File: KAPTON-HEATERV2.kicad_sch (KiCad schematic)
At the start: 21 parts, among them J1 XT60PW-M, J2 XT60PW-M, J3 1985276, J4 1985218, J5 10090926-P154XLF, K1 1-1393210-8, Q1 AO3400A, U1 TC4427ACOA

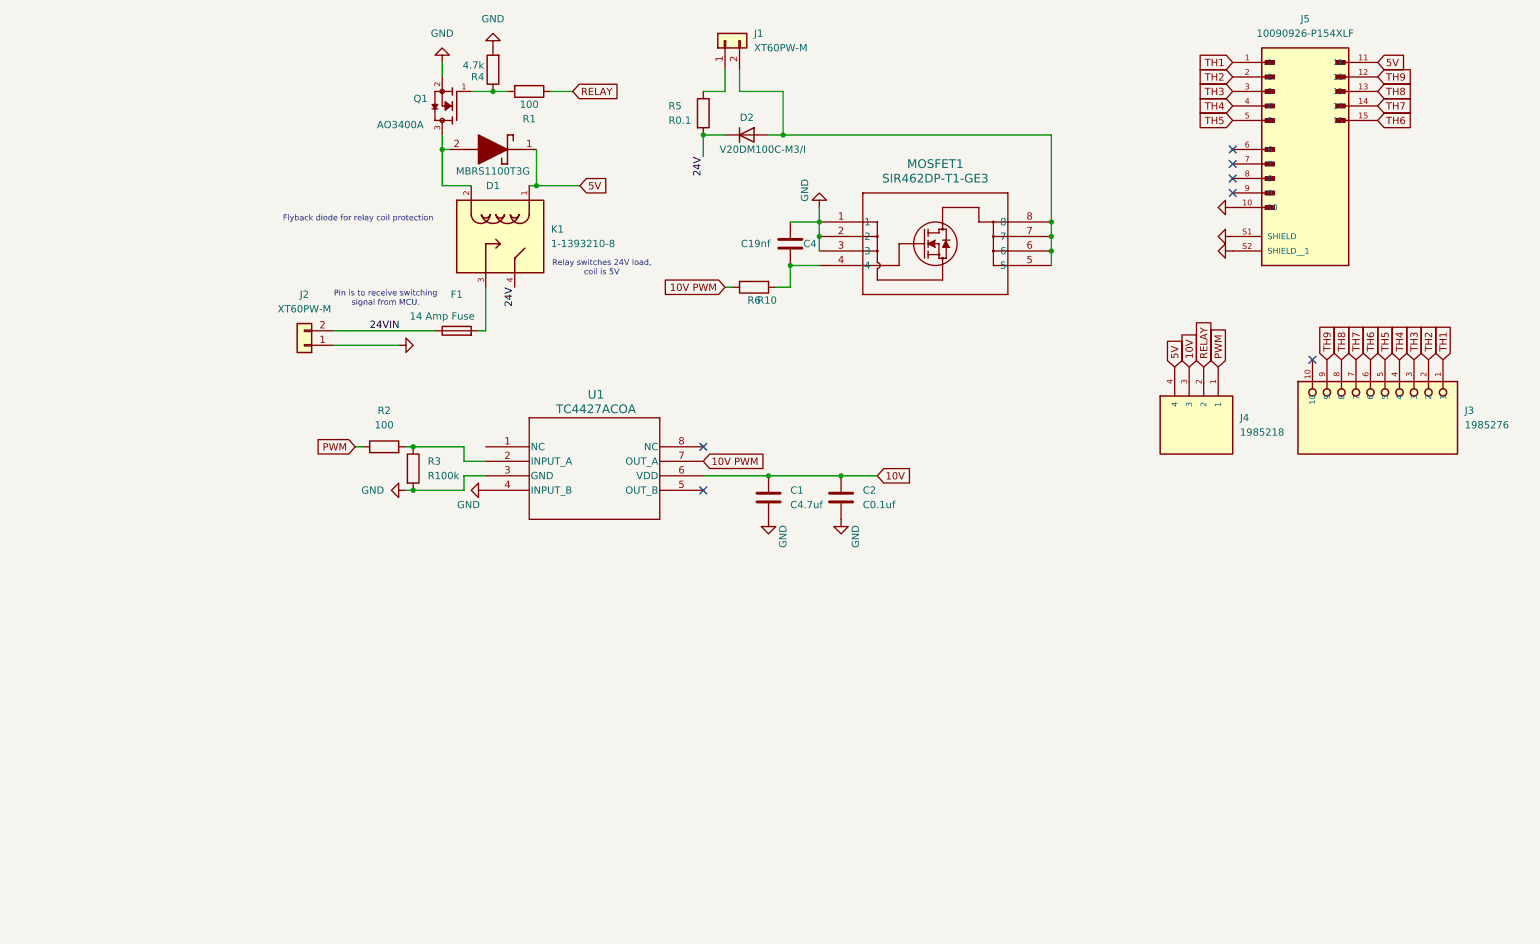
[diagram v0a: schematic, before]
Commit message: working on pcb
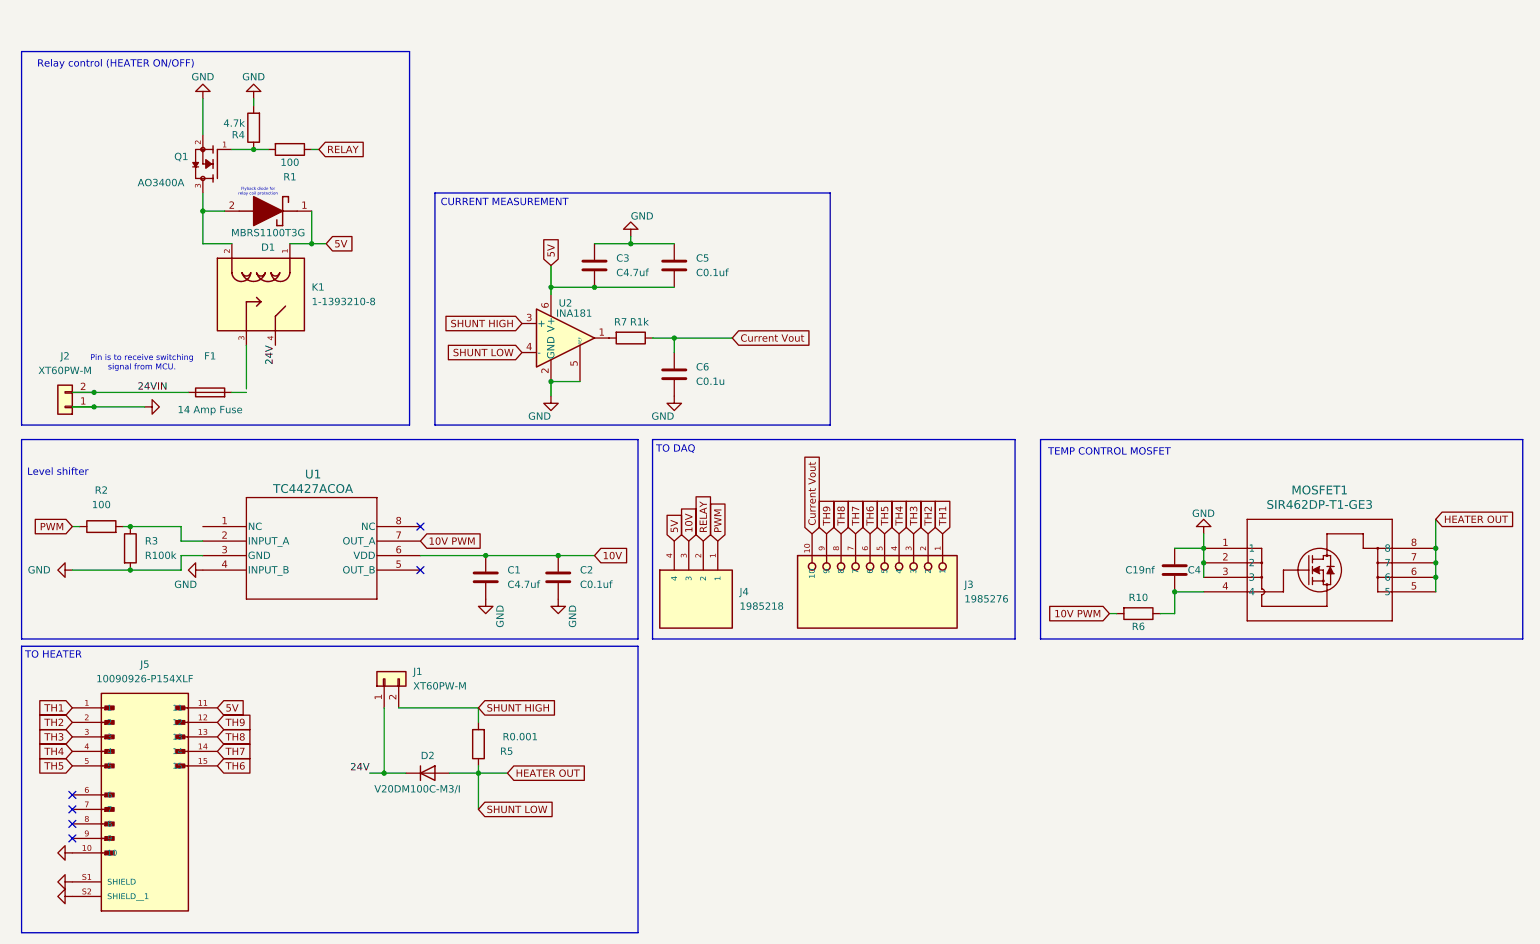
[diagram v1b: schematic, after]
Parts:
- added C3: C4.7uf, Capacitor_SMD:C_0805_2012Metric, symbol Device:C
- added C5: C0.1uf, Capacitor_SMD:C_0805_2012Metric, symbol Device:C
- added C6: C0.1u, Capacitor_SMD:C_0805_2012Metric, symbol Device:C
- added R7: R1k, Resistor_SMD:R_0805_2012Metric, symbol Device:R
- added U2: INA181, Package_TO_SOT_SMD:SOT-23-6, symbol Amplifier_Current:INA181
- R1, R2, R4, R6: footprint PCM_JLCPCB:R_1206 -> Resistor_SMD:R_0805_2012Metric
- R5: value R0.1 -> R0.001; footprint PCM_JLCPCB:R_1206 -> CRE2512_FZ_R001E_2 (1):RESC6432X90N
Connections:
- net 24V: now also J1.1 (Pin_1); no longer R5.2
- net 5V: now also C3.2, C5.2, U2.6 (V+)
- net GND: now also C3.1, C5.1, C6.2, U2.2 (GND), U2.5 (REF)
- net HEATER OUT: now reaches D2.2 (A), MOSFET1.5, MOSFET1.6, MOSFET1.7, MOSFET1.8
- net HEATER OUT: now also R5.1, U2.4 (-); no longer J1.2 (Pin_2)
- net Current Vout: now reaches J3.10
- net Current Vout: now also C6.1, R7.1
- net at K1.3: no longer F1.2
- new net: R7.2, U2.1
- new net SHUNT HIGH: J1.2 (Pin_2), R5.2, U2.3 (+)
- no-connect marks 7 -> 6
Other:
- note added: "CURRENT MEASUREMENT"
- note added: "Level shifter"
- note added: "Relay control (HEATER ON/OFF)"
- note added: "TEMP CONTROL MOSFET"
- note added: "TO DAQ"
- note added: "TO HEATER"
- note removed: "Relay switches 24V load, coil is 5V"
- moved on the sheet: C1, C2, C4, D1, D2, F1, J1, J2, J3, J4, J5, K1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
